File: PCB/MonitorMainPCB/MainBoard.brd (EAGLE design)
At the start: 94.1 x 100 mm, 147 parts, among them IC1 ADS1293, IC2 LP3878MR-ADJ_NOPB, J1 POWER_JACK, J2 USB_B_PTH, J6 2X6 FEMALE, U2 TPS7A4901DGNR, U3 AFE4400_RHA_40, U4 MSP430F149IPAG, Y1 4.096MHz, Y2 8MHz, Y3 12MHz, Y4 32.768kHz, Y5 8MHz

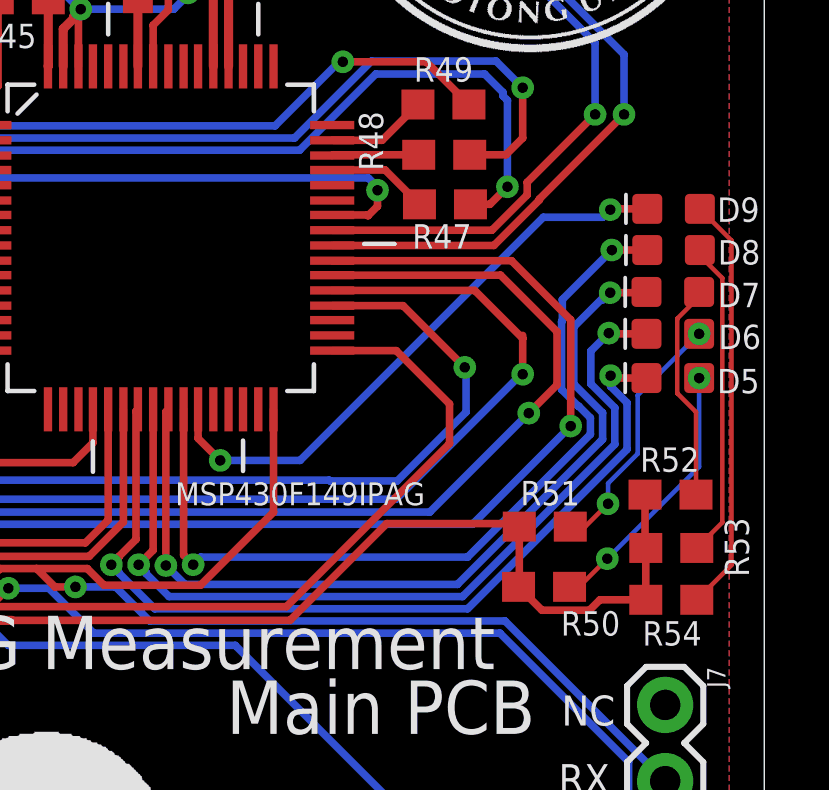
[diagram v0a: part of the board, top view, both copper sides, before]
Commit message: update some kind of mianPCB
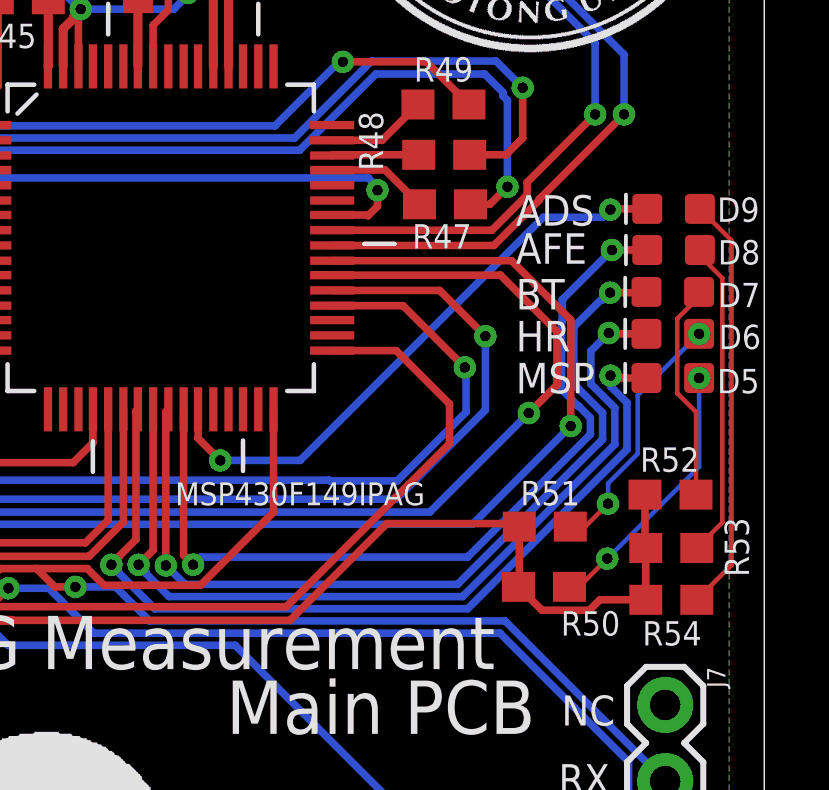
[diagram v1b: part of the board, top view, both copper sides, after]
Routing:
- net PD_ALM: track 80.9 -> 79.0 mm
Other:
- board text added: "ADS"
- board text added: "AFE"
- board text added: "BT"
- board text added: "HR"
- board text added: "MSP"
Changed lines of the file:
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@@
 <setting verticaltext="up"/>
 </settings>
-<grid distance="10" unitdist="mil" unit="mil" style="lines" multiple="1" display="yes" altdistance="5" altunitdist="mil" altunit="mil"/>
+<grid distance="5" unitdist="mil" unit="mil" style="lines" multiple="1" display="yes" altdistance="5" altunitdist="mil" altunit="mil"/>
 <layers>
 <layer number="1" name="Top" color="4" fill="1" visible="yes" active="yes"/>
@@
 <text x="26.6192" y="19.9644" size="1.016" layer="25" font="vector" ratio="20">U1</text>
 <text x="49.7332" y="60.3504" size="1.016" layer="21" font="vector" ratio="20">U5</text>
+<text x="85.852" y="70.993" size="1.016" layer="21" font="vector" ratio="20">ADS</text>
+<text x="85.852" y="69.723" size="1.016" layer="21" font="vector" ratio="20">AFE</text>
+<text x="85.852" y="68.199" size="1.016" layer="21" font="vector" ratio="20">BT</text>
+<text x="85.852" y="66.802" size="1.016" layer="21" font="vector" ratio="20">HR</text>
+<text x="85.852" y="65.405" size="1.016" layer="21" font="vector" ratio="20">MSP</text>
 </plain>
 <attributes>
@@
 <wire x1="58.293" y1="62.1382125" x2="59.2652125" y2="61.166" width="0.254" layer="16"/>
 <wire x1="58.293" y1="74.207425" x2="58.293" y2="62.1382125" width="0.254" layer="16"/>
-<wire x1="86.0298" y1="66.04" x2="86.0806" y2="66.04" width="0.254" layer="16"/>
-<via x="86.0806" y="66.04" extent="1-16" drill="0.35"/>
-<wire x1="86.0806" y1="66.04" x2="86.0806" y2="67.2338" width="0.254" layer="1"/>
-<wire x1="86.0806" y1="67.2338" x2="86.0806" y2="67.3354" width="0.254" layer="1"/>
 <contactref element="U4" pad="37"/>
-<wire x1="86.0806" y1="67.2338" x2="84.4804" y2="68.834" width="0.254" layer="1"/>
-<wire x1="84.4804" y1="68.834" x2="79.7306" y2="68.834" width="0.254" layer="1"/>
 <wire x1="59.484" y1="61.166" x2="59.9214" y2="61.166" width="0.254" layer="16"/>
 <wire x1="59.9214" y1="61.166" x2="60.6298" y2="61.8744" width="0.254" layer="16"/>
@@
 <wire x1="64.3706125" y1="61.8518" x2="64.9153875" y2="61.8518" width="0.254" layer="16"/>
 <wire x1="64.9153875" y1="61.8518" x2="64.9379875" y2="61.8744" width="0.254" layer="16"/>
-<wire x1="81.8642" y1="61.8744" x2="86.0298" y2="66.04" width="0.254" layer="16"/>
 <wire x1="64.9379875" y1="61.8744" x2="81.8642" y2="61.8744" width="0.254" layer="16"/>
+<wire x1="81.8642" y1="61.8744" x2="84.836" y2="64.8462" width="0.254" layer="16"/>
+<via x="84.836" y="67.31" extent="1-16" drill="0.35"/>
+<wire x1="84.836" y1="64.8462" x2="84.836" y2="67.31" width="0.254" layer="16"/>
+<wire x1="79.7306" y1="68.834" x2="83.312" y2="68.834" width="0.254" layer="1"/>
+<wire x1="83.312" y1="68.834" x2="84.836" y2="67.31" width="0.254" layer="1"/>
 </signal>
 <signal name="ADC_RDY">
@@
 <wire x1="81.8642" y1="66.8274" x2="83.6422" y2="65.0494" width="0.254" layer="1"/>
 <wire x1="83.6422" y1="65.0494" x2="83.6422" y2="63.7286" width="0.254" layer="1"/>
-<wire x1="78.2066" y1="58.293" x2="83.6422" y2="63.7286" width="0.254" layer="1"/>
+<wire x1="78.2066" y1="58.293" x2="81.8388" y2="61.9252" width="0.254" layer="1"/>
+<wire x1="81.8388" y1="61.9252" x2="83.6422" y2="63.7286" width="0.254" layer="1"/>
 <wire x1="64.611125" y1="58.293" x2="67.4116" y2="58.293" width="0.254" layer="1"/>
 <contactref element="J7" pad="3"/>
